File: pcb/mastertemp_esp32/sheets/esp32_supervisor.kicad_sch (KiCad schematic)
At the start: 5 parts, among them U4 WATCHDOG_SUPERVISOR_TBD, U5 ESP32-WROOM-32E-N16_CANDIDATE, U9 RELAY_GATE_LOGIC_TBD

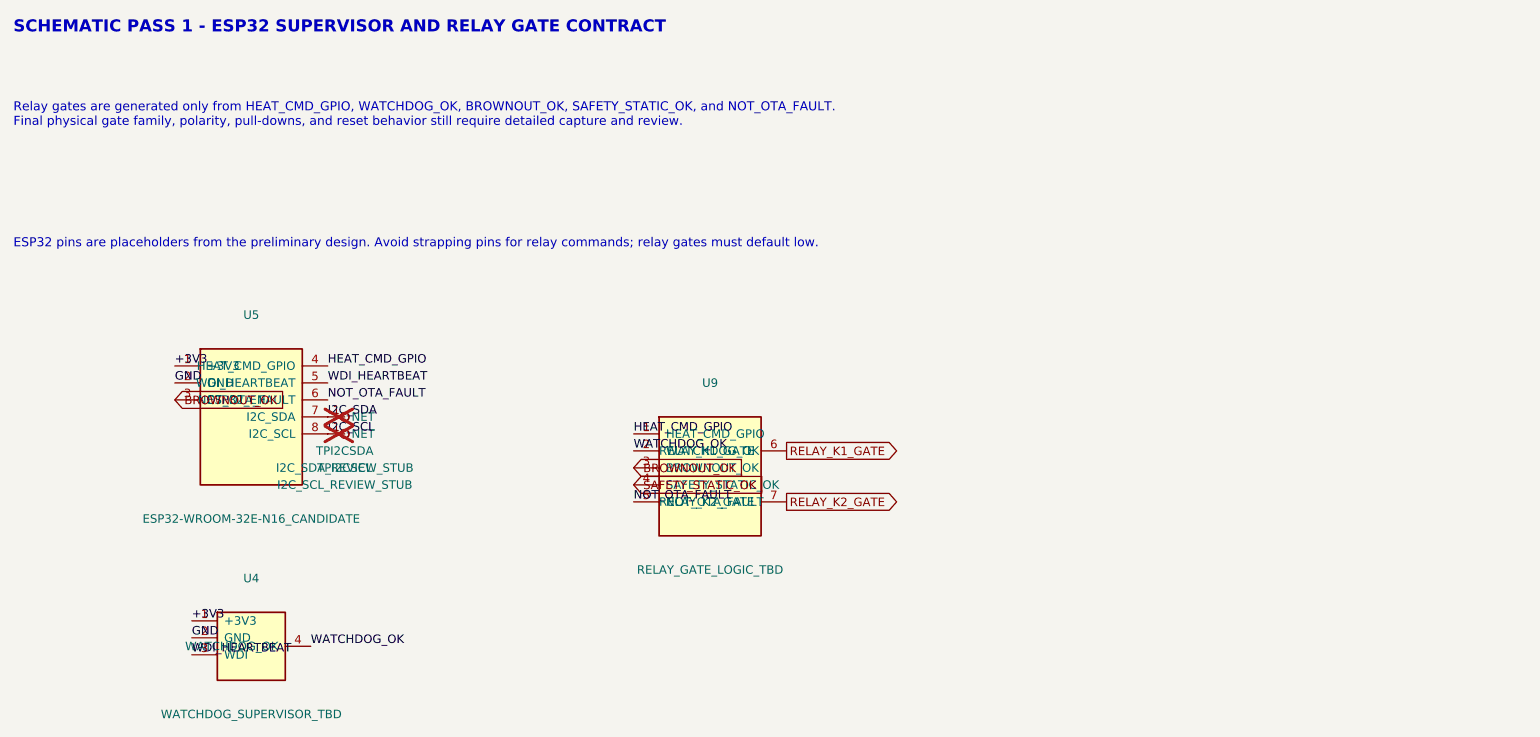
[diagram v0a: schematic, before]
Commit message: AI
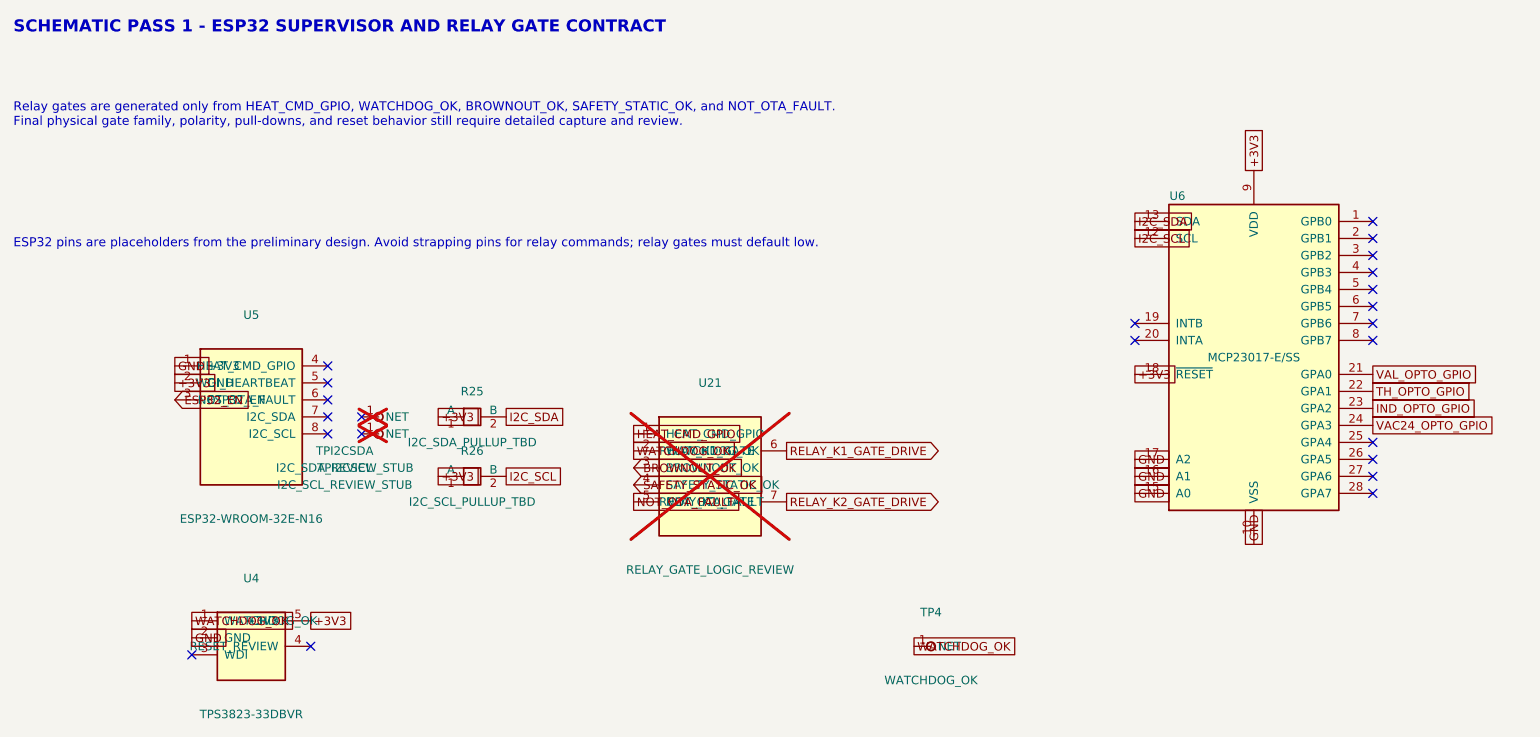
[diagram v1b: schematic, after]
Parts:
- added R25: I2C_SDA_PULLUP_TBD, Resistor_SMD:R_0805_2012Metric, symbol mastertemp_esp32:Resistor_2pin
- added R26: I2C_SCL_PULLUP_TBD, Resistor_SMD:R_0805_2012Metric, symbol mastertemp_esp32:Resistor_2pin
- added TP4: WATCHDOG_OK, TestPoint_Pad_D2.0mm, symbol mastertemp_esp32:NetStub_1pin
- added U6: MCP23017-E/SS, Package_SO:SSOP-28_5.3x10.2mm_P0.65mm, symbol mastertemp_esp32:MCP23017_SS
- U21: renamed from U9; value RELAY_GATE_LOGIC_TBD -> RELAY_GATE_LOGIC_REVIEW; now not fitted; now left out of the parts list
- U4: value WATCHDOG_SUPERVISOR_TBD -> TPS3823-33DBVR
- U5: value ESP32-WROOM-32E-N16_CANDIDATE -> ESP32-WROOM-32E-N16; footprint RF_Module:ESP32-WROOM-32 -> ESP32-WROOM-32E
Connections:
- net +3V3: now also U4.5 (+3V3), U5.2 (GND), R25.1 (A), R26.1 (A), U6.18 (~{RESET}), U6.9 (VDD); no longer U4.1 (+3V3), U5.1 (+3V3)
- net BROWNOUT_OK: no longer U5.3 (ESP32_EN)
- net GND: now also U5.1 (+3V3), U6.10 (VSS), U6.15 (A0), U6.16 (A1), U6.17 (A2); no longer U5.2 (GND)
- net HEAT_CMD_GPIO: no longer U5.4 (HEAT_CMD_GPIO)
- net I2C_SCL: now also R26.2 (B), U6.12 (SCL); no longer TPI2CSCL.1 (NET), U5.8 (I2C_SCL)
- net I2C_SDA: now also R25.2 (B), U6.13 (SDA); no longer TPI2CSDA.1 (NET), U5.7 (I2C_SDA)
- net NOT_OTA_FAULT: no longer U5.6 (NOT_OTA_FAULT)
- net WATCHDOG_OK: now also U4.1 (WATCHDOG_OK), TP4.1 (NET); no longer U4.4 (WATCHDOG_OK)
- net RELAY_K1_GATE renamed RELAY_K1_GATE_DRIVE
- net RELAY_K2_GATE renamed RELAY_K2_GATE_DRIVE
- net WDI_HEARTBEAT: no longer names the net of U4.3 (WDI)
- net WDI_HEARTBEAT: no longer U5.5 (WDI_HEARTBEAT)
- new net ESP32_EN: U5.3 (ESP32_EN)
- new net IND_OPTO_GPIO: U6.23 (GPA2)
- new net TH_OPTO_GPIO: U6.22 (GPA1)
- new net VAC24_OPTO_GPIO: U6.24 (GPA3)
- new net VAL_OPTO_GPIO: U6.21 (GPA0)
- no-connect marks 0 -> 23
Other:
- moved on the sheet: TPI2CSCL, TPI2CSDA
